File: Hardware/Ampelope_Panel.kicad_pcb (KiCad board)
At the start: 2 copper layers, 60.8 x 128.5 mm, 37 parts

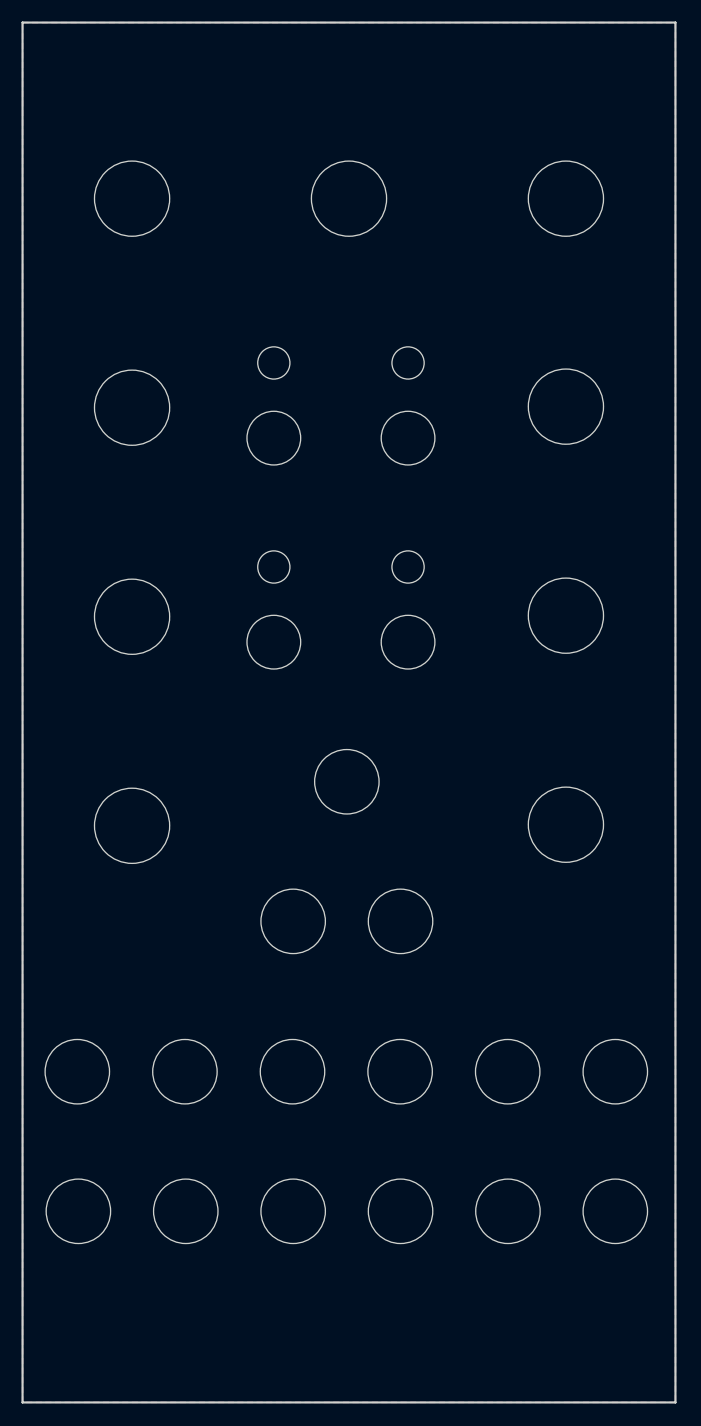
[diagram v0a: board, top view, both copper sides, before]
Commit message: Work on panel and control layout
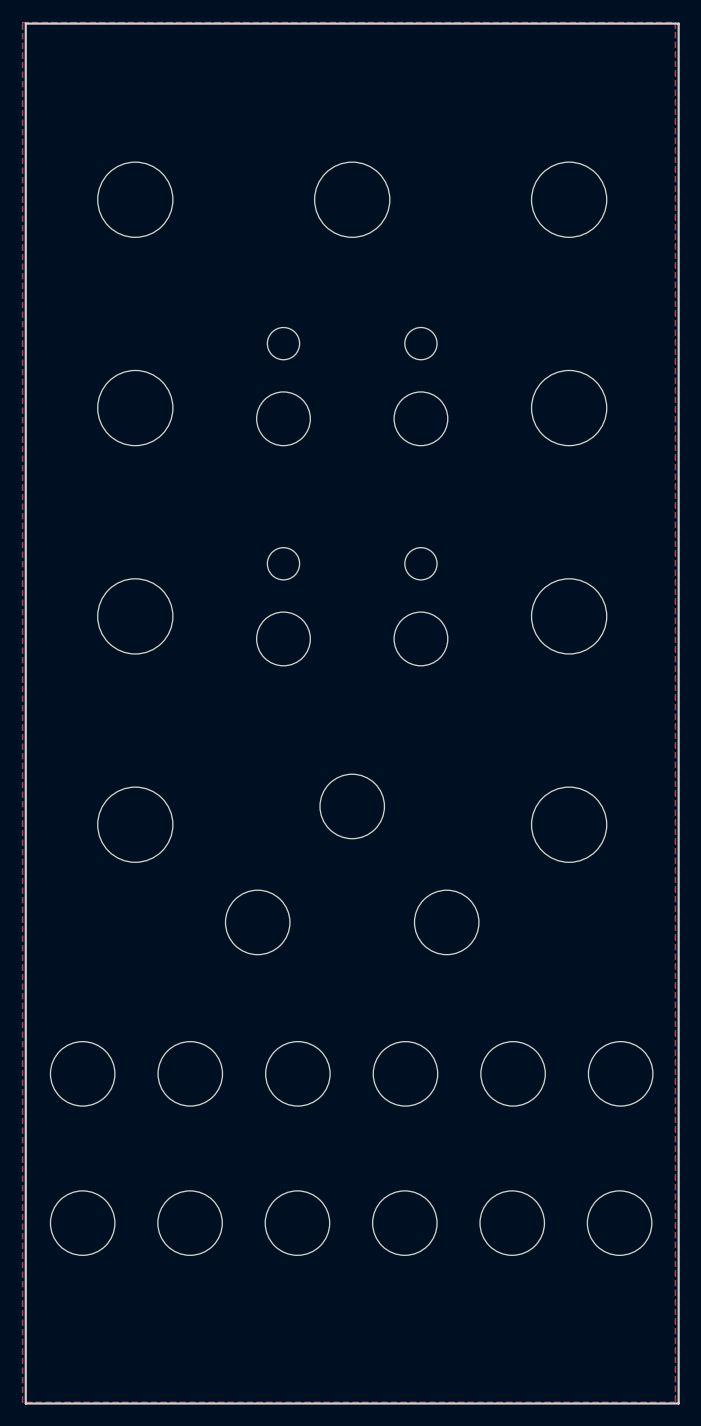
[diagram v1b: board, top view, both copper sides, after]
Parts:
- removed the G*** at (129.5, 44.9)
- added G***: LOGO, Logo_Footprint:logo, F.Cu at (130.3, 45.2)
- moved Ref** 4.30 mm to (139.1, 124.6)
- moved Ref** 3.30 mm to (121.5, 124.6)
- moved Ref** 2.35 mm to (130.3, 113.8)
- moved Ref** 2.16 mm to (136.7, 70.7)
- moved TYPE 2.16 mm to (136.7, 77.7)
- moved LED_L 2.01 mm to (123.9, 70.7)
- moved TYPE 2.01 mm to (123.9, 77.7)
- moved LED_L 1.24 mm to (136.7, 91.2)
- moved TYPE 1.24 mm to (136.7, 98.2)
- moved Ref** 1.17 mm to (125.2, 152.6)
- moved Ref** 1.17 mm to (105.2, 152.6)
- moved Ref** 1.17 mm to (115.2, 152.6)
- moved Ref** 1.17 mm to (145.2, 152.6)
- moved Ref** 1.17 mm to (155.2, 152.6)
- moved Ref** 1.17 mm to (135.2, 152.6)
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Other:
- board text added: "1"
- board text added: "2"
- board text added: "3"
- board text added: "4"
- board text added: "A"
- board text added: "D"
- board text added: "Env Out"
- board text added: "Gate"
- board text added: "LFO"
- board text added: "S"
- board text added: "T"
- board text removed: "Chorus"
- board text removed: "Del L"
- board text removed: "Del R"
- board text removed: "Delay L"
- board text removed: "Delay R"
- board text removed: "Dry/Wet"
- board text removed: "Feedback"
- board text removed: "Filter"
- board text removed: "HP"
- board text removed: "LP"
- board text removed: "Link"
- board text removed: "Reset"
- board text removed: "Reverse"
- board text removed: "Short"
- board text removed: "Wide"
